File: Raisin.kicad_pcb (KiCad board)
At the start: 2 copper layers, 6 parts, among them U1 ATMEGA328P-AU, U10 L78L06_TO92, U5 LD1117S33TR_SOT223, U6 L78L05_TO92, U7 FSA3157L6X, U8 AD5171

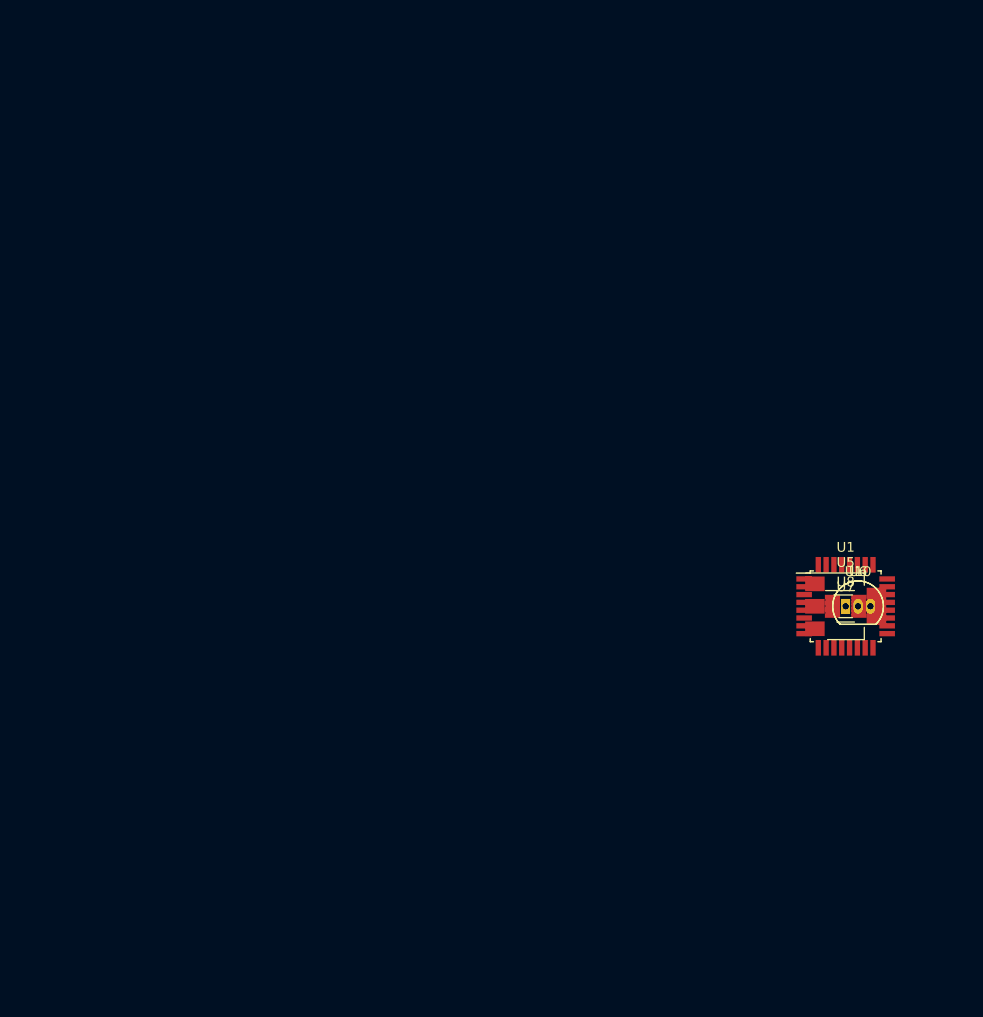
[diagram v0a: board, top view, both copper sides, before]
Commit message: bad pcb layout
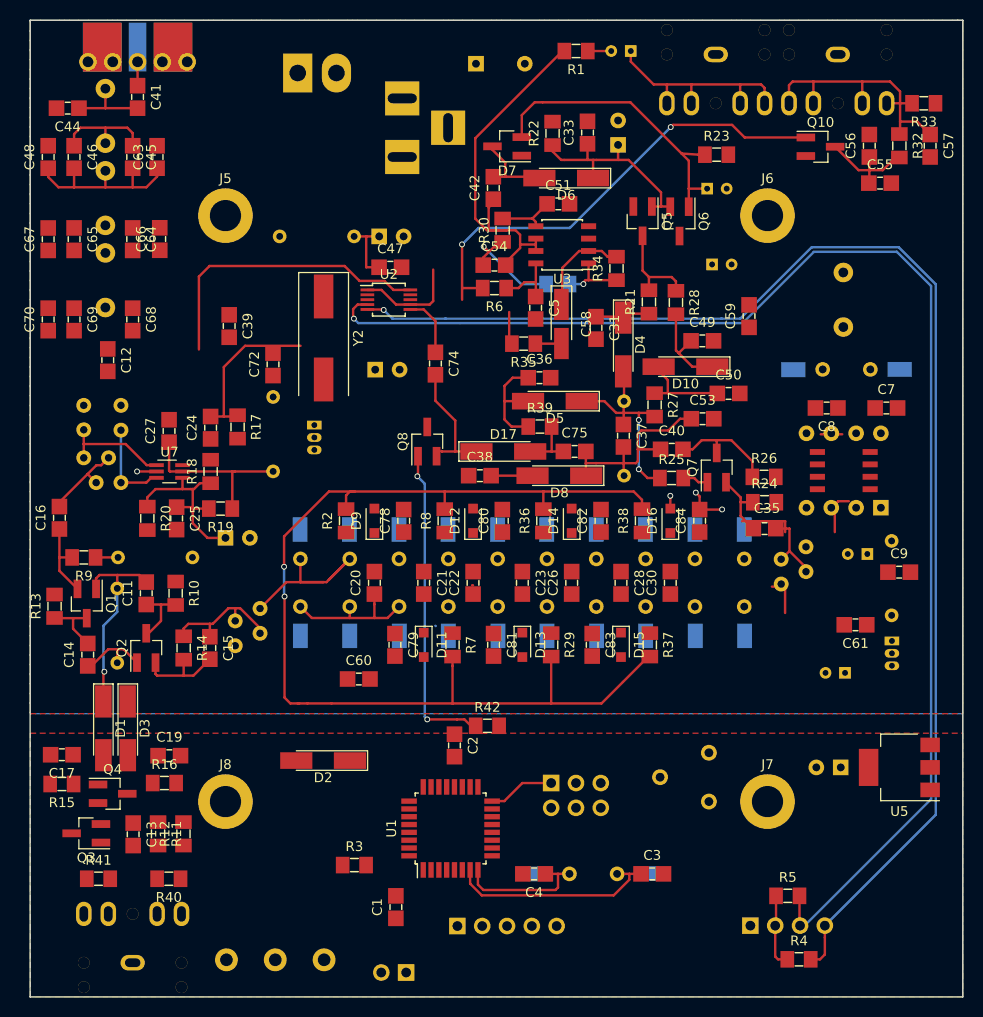
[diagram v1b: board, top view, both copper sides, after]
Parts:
- removed U8: AD5171, TO_SOT_Packages_SMD:SOT-23-8_Handsoldering
- added C1: 100nF, raisin:C_1206_0603, F.Cu at (102.5, 135.8)
- added C10: 10uF, Capacitors_ThroughHole:CP_Radial_D4.0mm_P2.00mm, B.Cu at (150.7, 99.7)
- added C11: 10nF, raisin:C_1206_0603, F.Cu at (76.9, 103.7)
- added C12: 10nF, raisin:C_1206_0603, F.Cu at (73.0, 79.8)
- added C13: 100nF, raisin:C_1206_0603, F.Cu at (75.5, 128.3)
- added C14: 10nF, raisin:C_1206_0603, F.Cu at (70.9, 110.0)
- added C15: 100nF, raisin:C_1206_0603, F.Cu at (83.4, 109.3)
- added C16: 10nF, raisin:C_1206_0603, F.Cu at (68.0, 95.9)
- added C17: 100nF, raisin:C_1206_0603, F.Cu at (68.2, 120.2)
- added C19: 100nF, raisin:C_1206_0603, F.Cu at (79.2, 120.3)
- added C2: 100nF, raisin:C_1206_0603, F.Cu at (108.5, 119.2)
- added C20: 220nF, raisin:C_1206_0603, F.Cu at (100.2, 102.6)
- added C21: 220nF, raisin:C_1206_0603, F.Cu at (105.3, 102.6)
- added C22: 220nF, raisin:C_1206_0603, F.Cu at (110.3, 102.6)
- added C23: 220nF, raisin:C_1206_0603, F.Cu at (115.4, 102.6)
- added C24: 10nF, raisin:C_1206_0603, F.Cu at (83.5, 86.7)
- added C25: 100nF, raisin:C_1206_0603, F.Cu at (80.0, 96.0)
- added C26: 220nF, raisin:C_1206_0603, F.Cu at (120.5, 102.6)
- added C27: 100nF, raisin:C_1206_0603, F.Cu at (79.2, 87.0)
- added C28: 220nF, raisin:C_1206_0603, F.Cu at (125.5, 102.6)
- added C29: 33uF, Capacitors_ThroughHole:CP_Radial_D6.3mm_P2.50mm, B.Cu at (85.0, 98.0)
- added C3: 22pF, raisin:C_1206_0603, F.Cu at (128.7, 132.4)
- added C30: 220nF, raisin:C_1206_0603, F.Cu at (130.6, 102.6)
- added C31: 100nF, raisin:C_1206_0603, F.Cu at (122.9, 76.5)
- added C32: 33uF, Capacitors_ThroughHole:CP_Radial_D6.3mm_P2.50mm, B.Cu at (125.2, 57.8)
- added C33: 100nF, raisin:C_1206_0603, F.Cu at (122.1, 56.5)
- added C34: 1uF, Capacitors_ThroughHole:CP_Radial_D4.0mm_P2.00mm, B.Cu at (134.3, 62.2)
- added C35: 100nF, raisin:C_1206_0603, F.Cu at (140.2, 97.0)
- added C36: 100nF, raisin:C_1206_0603, F.Cu at (117.2, 81.6)
- added C37: 75*, raisin:C_1206_0603, F.Cu at (125.8, 87.5)
- added C38: 100nF, raisin:C_1206_0603, F.Cu at (111.0, 91.6)
- added C39: 10nF, raisin:C_1206_0603, F.Cu at (85.4, 76.3)
- added C4: 22pF, raisin:C_1206_0603, F.Cu at (116.6, 132.4)
- added C40: 10nF, raisin:C_1206_0603, F.Cu at (130.7, 88.9)
- added C41: 10nF, raisin:C_1206_0603, F.Cu at (76.0, 52.9)
- added C42: 100nF, raisin:C_1206_0603, F.Cu at (112.4, 62.2)
- added C43: 1uF, Capacitors_ThroughHole:CP_Radial_D4.0mm_P2.00mm, B.Cu at (126.5, 48.1)
- added C44: 270, raisin:C_1206_0603, F.Cu at (68.8, 54.0)
- added C45: 27, raisin:C_1206_0603, F.Cu at (75.5, 59.0)
- added C46: 33, raisin:C_1206_0603, F.Cu at (69.5, 59.0)
- added C47: 100nF, raisin:C_1206_0603, F.Cu at (101.9, 70.3)
- added C48: 680, raisin:C_1206_0603, F.Cu at (66.8, 59.0)
- added C49: 100nF, raisin:C_1206_0603, F.Cu at (133.8, 77.8)
- added C5: 100nF, raisin:C_1206_0603, F.Cu at (116.8, 74.4)
- added C50: 10nF, raisin:C_1206_0603, F.Cu at (136.5, 83.2)
- added C51: 4n7, raisin:C_1206_0603, F.Cu at (119.1, 63.8)
- added C52: 10uF, Capacitors_ThroughHole:CP_Radial_D5.0mm_P2.50mm, B.Cu at (100.7, 67.1)
- added C53: 10nF, raisin:C_1206_0603, F.Cu at (133.8, 85.8)
- added C54: 47n, raisin:C_1206_0603, F.Cu at (112.5, 70.1)
- added C55: 100nF, raisin:C_1206_0603, F.Cu at (152.0, 61.7)
- added C56: 10nF, raisin:C_1206_0603, F.Cu at (150.9, 57.9)
- added C57: 10nF, raisin:C_1206_0603, F.Cu at (157.2, 57.9)
- added C58: 10uF, Capacitors_Tantalum_SMD:CP_Tantalum_Case-A_EIA-3216-18_Hand, F.Cu at (119.4, 76.1)
- added C59: 10nF, raisin:C_1206_0603, F.Cu at (138.6, 75.3)
- added C60: 100nF, raisin:C_1206_0603, F.Cu at (98.7, 112.5)
- added C61: 100nF, raisin:C_1206_0603, F.Cu at (149.5, 106.9)
- added C62: 10uF, Capacitors_ThroughHole:CP_Radial_D4.0mm_P2.00mm, B.Cu at (148.4, 111.8)
- added C63: 22, raisin:C_1206_0603, F.Cu at (78.0, 59.0)
- added C64: 27, raisin:C_1206_0603, F.Cu at (75.5, 67.4)
- added C65: 33, raisin:C_1206_0603, F.Cu at (69.5, 67.4)
- added C66: 680, raisin:C_1206_0603, F.Cu at (78.3, 67.4)
- added C67: 22, raisin:C_1206_0603, F.Cu at (66.8, 67.4)
- added C68: 27, raisin:C_1206_0603, F.Cu at (75.5, 75.6)
- added C69: 33, raisin:C_1206_0603, F.Cu at (69.5, 75.6)
- added C7: 22pF, raisin:C_1206_0603, F.Cu at (152.7, 84.7)
- added C70: 270, raisin:C_1206_0603, F.Cu at (66.8, 75.6)
- added C71: 1uF, Capacitors_ThroughHole:CP_Radial_D4.0mm_P2.00mm, B.Cu at (134.8, 70.0)
- added C72: 100nF, raisin:C_1206_0603, F.Cu at (89.9, 80.2)
- added C73: 33uF, Capacitors_ThroughHole:CP_Radial_D6.3mm_P2.50mm, B.Cu at (100.3, 80.8)
- added C74: 10nF, raisin:C_1206_0603, F.Cu at (106.5, 80.2)
- added C75: 10nF, raisin:C_1206_0603, F.Cu at (120.8, 89.2)
- added C76: 330uF, Capacitors_ThroughHole:CP_Radial_D8.0mm_P5.00mm, B.Cu at (110.7, 49.5)
- added C77: 100uF, Capacitors_ThroughHole:CP_Radial_D6.3mm_P2.50mm, B.Cu at (148.0, 121.5)
- added C78: 100pF, raisin:C_1206_0603, F.Cu at (103.2, 96.2)
- added C79: 100pF, raisin:C_1206_0603, F.Cu at (102.3, 109.0)
- added C8: 22pF, raisin:C_1206_0603, F.Cu at (146.6, 84.7)
- added C80: 100pF, raisin:C_1206_0603, F.Cu at (113.3, 96.2)
- added C81: 100pF, raisin:C_1206_0603, F.Cu at (112.5, 109.0)
- added C82: 100pF, raisin:C_1206_0603, F.Cu at (123.5, 96.2)
- added C83: 100pF, raisin:C_1206_0603, F.Cu at (122.5, 109.0)
- added C84: 100pF, raisin:C_1206_0603, F.Cu at (133.6, 96.2)
- added C9: 100nF, raisin:C_1206_0603, F.Cu at (154.0, 101.5)
- added CON1: AVR_ISP, Pin_Headers:Pin_Header_Straight_2x03_Pitch2.54mm, B.Cu at (118.3, 123.1)
- added D1: LL4148, Diodes_SMD:D_MiniMELF_Handsoldering, F.Cu at (72.5, 117.5)
- added D10: LL4148, Diodes_SMD:D_MiniMELF_Handsoldering, F.Cu at (132.1, 80.5)
- added D11: BB132, Diodes_SMD:D_SOD-323_HandSoldering, F.Cu at (105.3, 109.0)
- added D12: BB132, Diodes_SMD:D_SOD-323_HandSoldering, F.Cu at (110.3, 96.2)
- added D13: BB132, Diodes_SMD:D_SOD-323_HandSoldering, F.Cu at (115.4, 109.0)
- added D14: BB132, Diodes_SMD:D_SOD-323_HandSoldering, F.Cu at (120.5, 96.2)
- added D15: BB132, Diodes_SMD:D_SOD-323_HandSoldering, F.Cu at (125.5, 109.0)
- added D16: BB132, Diodes_SMD:D_SOD-323_HandSoldering, F.Cu at (130.6, 96.2)
- added D17: LL4148, Diodes_SMD:D_MiniMELF_Handsoldering, F.Cu at (113.5, 89.2)
- added D2: LL4148, Diodes_SMD:D_MiniMELF_Handsoldering, F.Cu at (95.0, 120.8)
- added D3: LL4148, Diodes_SMD:D_MiniMELF_Handsoldering, F.Cu at (75.0, 117.5)
- added D4: LL4148, Diodes_SMD:D_MiniMELF_Handsoldering, F.Cu at (125.7, 78.2)
- added D5: LL4148, Diodes_SMD:D_MiniMELF_Handsoldering, F.Cu at (118.7, 84.0)
- added D6: LL4148, Diodes_SMD:D_MiniMELF_Handsoldering, F.Cu at (119.9, 61.2)
- added D7: BAV99, TO_SOT_Packages_SMD:SOT-23_Handsoldering, F.Cu at (113.8, 57.9)
- added D8: LL4148, Diodes_SMD:D_MiniMELF_Handsoldering, F.Cu at (119.2, 91.6)
- added D9: BB132, Diodes_SMD:D_SOD-323_HandSoldering, F.Cu at (100.2, 96.2)
- added J1: PTT, Socket_Strips:Socket_Strip_Angled_1x02_Pitch2.54mm, B.Cu at (103.5, 142.5)
- added J10: Conn_01x05, Pin_Headers:Pin_Header_Straight_1x05_Pitch2.54mm, B.Cu at (108.8, 137.7)
- added J11: i2c, raisin:SSD1306, B.Cu at (142.5, 137.7)
- added J12: Barrel_Jack, Connect:BARREL_JACK, B.Cu at (103.1, 59.0)
- added J13: PA, Connectors_Molex:Molex_KK-41791-02_02x3.96mm_Straight, B.Cu at (92.4, 50.4)
- added J2: Line OUT, raisin:audio_jack_3_5mm_PJ307, B.Cu at (135.2, 48.5)
- added J3: MIC, raisin:audio_jack_3_5mm_PJ307, B.Cu at (147.7, 48.5)
- added J4: ANT_PA, raisin:RFCONNECTOR, B.Cu at (76.0, 50.4)
- added J5: Conn_01x01, Mounting_Holes:MountingHole_3.2mm_M3_DIN965_Pad, F.Cu at (85.0, 65.0)
- added J6: Conn_01x01, Mounting_Holes:MountingHole_3.2mm_M3_DIN965_Pad, F.Cu at (140.5, 65.0)
- added J7: Conn_01x01, Mounting_Holes:MountingHole_3.2mm_M3_DIN965_Pad, F.Cu at (140.5, 125.0)
- added J8: Conn_01x01, Mounting_Holes:MountingHole_3.2mm_M3_DIN965_Pad, F.Cu at (85.0, 125.0)
- added J9: KEY, raisin:audio_jack_3_5mm_PJ307, B.Cu at (75.5, 141.5)
- added L1: L_Small, raisin:Choke_Toroid_6,5x13mm_Vertical, B.Cu at (154.9, 76.9)
- added L10: 8.5uH, raisin:Choke_Toroid_6,5x13mm_Vertical, B.Cu at (66.1, 59.9)
- added L11: 8.5uH, raisin:Choke_Toroid_6,5x13mm_Vertical, B.Cu at (66.1, 68.3)
- added L2: 47uH, Resistors_ThroughHole:R_Axial_DIN0204_L3.6mm_D1.6mm_P7.62mm_Horizontal, B.Cu at (153.2, 105.9)
- added L3: 22uH, Resistors_ThroughHole:R_Axial_DIN0204_L3.6mm_D1.6mm_P7.62mm_Horizontal, B.Cu at (81.6, 100.0)
- added L4: 22uH, Resistors_ThroughHole:R_Axial_DIN0204_L3.6mm_D1.6mm_P7.62mm_Horizontal, B.Cu at (73.9, 103.2)
- added L5: 47uH, Resistors_ThroughHole:R_Axial_DIN0204_L3.6mm_D1.6mm_P7.62mm_Horizontal, B.Cu at (89.9, 83.6)
- added L6: 47uH, Resistors_ThroughHole:R_Axial_DIN0204_L3.6mm_D1.6mm_P7.62mm_Horizontal, B.Cu at (90.5, 67.1)
- added L7: 22uH, Resistors_ThroughHole:R_Axial_DIN0204_L3.6mm_D1.6mm_P7.62mm_Horizontal, B.Cu at (125.8, 84.0)
- added L8: 8.5uH, raisin:Choke_Toroid_6,5x13mm_Vertical, B.Cu at (66.1, 51.5)
- added Q1: MMBFJ310LT1G, TO_SOT_Packages_SMD:SOT-23_Handsoldering, F.Cu at (70.8, 104.7)
- added Q10: BSS138, TO_SOT_Packages_SMD:SOT-23_Handsoldering, F.Cu at (145.9, 58.0)
- added Q2: MMBFJ310LT1G, TO_SOT_Packages_SMD:SOT-23_Handsoldering, F.Cu at (76.9, 109.3)
- added Q3: Si2301-TP, TO_SOT_Packages_SMD:SOT-23_Handsoldering, F.Cu at (70.8, 128.2)
- added Q4: Si2301-TP, TO_SOT_Packages_SMD:SOT-23_Handsoldering, F.Cu at (73.5, 124.2)
- added Q5: 2N7002, TO_SOT_Packages_SMD:SOT-23_Handsoldering, F.Cu at (127.7, 65.6)
- added Q6: MMBT3906, TO_SOT_Packages_SMD:SOT-23_Handsoldering, F.Cu at (131.5, 65.6)
- added Q7: MMBFJ310LT1G, TO_SOT_Packages_SMD:SOT-23_Handsoldering, F.Cu at (135.3, 90.8)
- added Q8: 2N7002, TO_SOT_Packages_SMD:SOT-23_Handsoldering, F.Cu at (105.7, 88.1)
- added R1: 560, raisin:R_1206_0603, F.Cu at (120.9, 48.1)
- added R10: 10k, raisin:R_1206_0603, F.Cu at (79.9, 103.7)
- added R11: 2.7k, raisin:R_1206_0603, F.Cu at (78.1, 128.3)
- added R12: 2.7k, raisin:R_1206_0603, F.Cu at (80.7, 128.3)
- added R13: 10k, raisin:R_1206_0603, F.Cu at (67.5, 105.0)
- added R14: 30, raisin:R_1206_0603, F.Cu at (80.7, 109.3)
- added R15: 4.7k, raisin:R_1206_0603, F.Cu at (68.2, 123.2)
- added R16: 4.7k, raisin:R_1206_0603, F.Cu at (78.8, 123.1)
- added R17: 100, raisin:R_1206_0603, F.Cu at (86.2, 86.6)
- added R18: 100, raisin:R_1206_0603, F.Cu at (83.5, 91.2)
- added R19: 3,3k, raisin:R_1206_0603, F.Cu at (84.5, 95.0)
- added R2: 300k, raisin:R_1206_0603, F.Cu at (97.3, 96.2)
- added R20: 3,3k, raisin:R_1206_0603, F.Cu at (77.0, 96.0)
- added R21: 1k, raisin:R_1206_0603, F.Cu at (128.4, 73.8)
- added R22: 1M, raisin:R_1206_0603, F.Cu at (118.5, 56.6)
- added R23: 150k*, raisin:R_1206_0603, F.Cu at (135.3, 58.8)
- added R24: 30, raisin:R_1206_0603, F.Cu at (140.2, 94.3)
- added R25: 300*, raisin:R_1206_0603, F.Cu at (130.7, 91.9)
- added R26: 10k, raisin:R_1206_0603, F.Cu at (140.2, 91.8)
- added R27: 1k, raisin:R_1206_0603, F.Cu at (128.9, 84.4)
- added R28: 1k, raisin:R_1206_0603, F.Cu at (131.1, 73.9)
- added R29: 300k, raisin:R_1206_0603, F.Cu at (118.3, 109.0)
- added R3: 10k, raisin:R_1206_0603, F.Cu at (98.2, 131.5)
- added R30: 15k, raisin:R_1206_0603, F.Cu at (113.4, 66.5)
- added R31: 1k, raisin:R_1206_0603, B.Cu at (119.0, 72.0)
- added R32: 1k, raisin:R_1206_0603, F.Cu at (154.0, 57.9)
- added R33: 15k, raisin:R_1206_0603, F.Cu at (156.5, 53.5)
- added R34: 15k, raisin:R_1206_0603, F.Cu at (125.0, 70.4)
- added R35: 300*, raisin:R_1206_0603, F.Cu at (115.5, 78.1)
- added R36: 300k, raisin:R_1206_0603, F.Cu at (117.5, 96.2)
- added R37: 300k, raisin:R_1206_0603, F.Cu at (128.4, 109.0)
- added R38: 300k, raisin:R_1206_0603, F.Cu at (127.7, 96.2)
- added R39: 1k, raisin:R_1206_0603, F.Cu at (117.2, 86.6)
- added R4: 4.7k, raisin:R_1206_0603, F.Cu at (143.7, 141.2)
- added R40: 470k, raisin:R_1206_0603, F.Cu at (79.2, 132.9)
- added R41: 470k, raisin:R_1206_0603, F.Cu at (72.0, 132.9)
- added R42: 1k, raisin:R_1206_0603, F.Cu at (111.8, 117.2)
- added R5: 4.7k, raisin:R_1206_0603, F.Cu at (142.6, 134.7)
- added R6: 100, raisin:R_1206_0603, F.Cu at (112.5, 72.4)
- added R7: 300k, raisin:R_1206_0603, F.Cu at (108.2, 109.0)
- added R8: 300k, raisin:R_1206_0603, F.Cu at (107.5, 96.2)
- added R9: 30, raisin:R_1206_0603, F.Cu at (70.5, 100.0)
- added RV1: POT, raisin:Potentiometer_WH148, B.Cu at (95.1, 141.2)
- added RV2: POT, raisin:Potentiometer_Trimmer_Piher_PT-6v_Horizontal, B.Cu at (134.5, 125.0)
- added T1: 1:2, raisin:TF12, B.Cu at (70.5, 84.4)
- added T2: Transformer, raisin:TF14, B.Cu at (70.5, 89.8)
- added T3: Transformer, raisin:TF14, B.Cu at (86.0, 109.0)
- added T4: Transformer, raisin:TF14, B.Cu at (141.9, 102.7)
- added U2: Si5351, Housings_SSOP:MSOP-10_3x3mm_Pitch0.5mm, F.Cu at (101.7, 73.6)
- added U3: NE5532, Housings_SOIC:SOIC-8_3.9x4.9mm_Pitch1.27mm, F.Cu at (119.5, 68.0)
- added U4: SA612A, raisin:DIP-8_SOIC-8_W7.62mm, B.Cu at (152.1, 94.9)
- added Y1: 8Mhz, raisin:Crystal_HC49-U_Vertical, B.Cu at (125.1, 132.4)
- added Y10: Crystal_GND23_Small, raisin:Crystal_HC49-U_Vertical, B.Cu at (123.0, 105.0)
- added Y11: Crystal_GND23_Small, raisin:Crystal_HC49-U_Vertical, B.Cu at (128.0, 100.2)
- added Y12: Crystal_GND23_Small, raisin:Crystal_HC49-U_Vertical, B.Cu at (138.1, 105.0)
- added Y13: Crystal_GND23_Small, raisin:Crystal_HC49-U_Vertical, B.Cu at (133.1, 105.0)
- added Y2: 27Mhz, Crystals:Crystal_SMD_HC49-SD, F.Cu at (95.0, 77.5)
- added Y3: Crystal_GND23_Small, raisin:Crystal_HC49-U_Vertical, B.Cu at (146.2, 80.8)
- added Y4: Crystal_GND23_Small, raisin:Crystal_HC49-U_Vertical, B.Cu at (92.7, 100.2)
- added Y5: Crystal_GND23_Small, raisin:Crystal_HC49-U_Vertical, B.Cu at (97.7, 100.2)
- added Y6: Crystal_GND23_Small, raisin:Crystal_HC49-U_Vertical, B.Cu at (102.8, 105.0)
- added Y7: Crystal_GND23_Small, raisin:Crystal_HC49-U_Vertical, B.Cu at (107.8, 100.2)
- added Y8: Crystal_GND23_Small, raisin:Crystal_HC49-U_Vertical, B.Cu at (112.9, 105.0)
- added Y9: Crystal_GND23_Small, raisin:Crystal_HC49-U_Vertical, B.Cu at (117.9, 100.2)
- U10, U6: moved to B.Cu
- moved U7 70.6 mm to (79.3, 91.2)
- moved U6 57.5 mm to (94.1, 86.5), turned to 270 degrees
- moved U1 46.4 mm to (108.0, 127.8), turned to 90 degrees
- moved U5 17.4 mm to (154.0, 121.5), turned to 180 degrees
- moved U10 5.92 mm to (153.2, 108.5), turned to 270 degrees
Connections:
- U1 pad 1: (no net) -> Net-(J10-Pad2)
- U1 pad 10: (no net) -> Net-(R40-Pad2)
- U1 pad 13: (no net) -> Net-(J1-Pad1)
- U1 pad 14: (no net) -> TONE
- U1 pad 15: (no net) -> KEY
- U1 pad 16: (no net) -> PTT
- U1 pad 17: (no net) -> Net-(CON1-Pad3)
- U1 pad 19: (no net) -> Net-(J10-Pad3)
- U1 pad 2: (no net) -> Net-(J9-Pad2)
- U1 pad 20: (no net) -> Net-(C2-Pad2)
- U1 pad 22: (no net) -> Net-(RV2-Pad2)
- U1 pad 29: (no net) -> Net-(CON1-Pad5)
- U1 pad 32: (no net) -> Net-(J10-Pad1)
- U1 pad 7: (no net) -> Net-(C3-Pad1)
- U1 pad 8: (no net) -> Net-(C4-Pad1)
- U1 pad 9: (no net) -> Net-(J9-Pad1)
- U10 pad 1: (no net) -> Net-(C61-Pad1)
- U6 pad 1: (no net) -> Net-(C72-Pad1)
- U7 pad 1: (no net) -> Net-(T1-Pad3)
- U7 pad 3: (no net) -> Net-(T1-Pad4)
- U7 pad 4: (no net) -> Net-(C25-Pad1)
- U7 pad 5: (no net) -> Net-(C27-Pad1)
- U7 pad 6: (no net) -> Net-(C24-Pad1)
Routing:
- net SCL: track 0.00 -> 140.8 mm, vias 0 -> 1
- net SDA: track 0.00 -> 138.2 mm, vias 0 -> 1
- net Net-(C60-Pad1): track 0.00 -> 111.8 mm, vias 0 -> 2
- net RX: track 0.00 -> 52.8 mm, vias 0 -> 2
- net Net-(C42-Pad1): track 0.00 -> 38.1 mm
- net Net-(Q8-Pad1): track 0.00 -> 32.6 mm, vias 0 -> 2
- net Net-(C34-Pad1): track 0.00 -> 31.3 mm
- net Net-(C39-Pad1): track 0.00 -> 30.6 mm
- net Net-(C57-Pad1): track 0.00 -> 28.9 mm
- net Net-(C43-Pad1): track 0.00 -> 23.3 mm
- net Net-(C37-Pad1): track 0.00 -> 22.5 mm, vias 0 -> 2
- net AGC_OFF: track 0.00 -> 22.2 mm
- net Net-(C37-Pad2): track 0.00 -> 22.1 mm
- net Net-(C3-Pad1): track 0.00 -> 21.9 mm
- net Net-(C11-Pad2): track 0.00 -> 20.3 mm, vias 0 -> 1
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- added copper zone on B.Cu, net GND
- added copper zone on F.Cu, net GND
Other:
- board outline added: 95.5 x 100 mm
